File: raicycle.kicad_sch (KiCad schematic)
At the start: 8 parts, among them U1 ESP32_Feather, U2 VL53L0X, U3 BME688

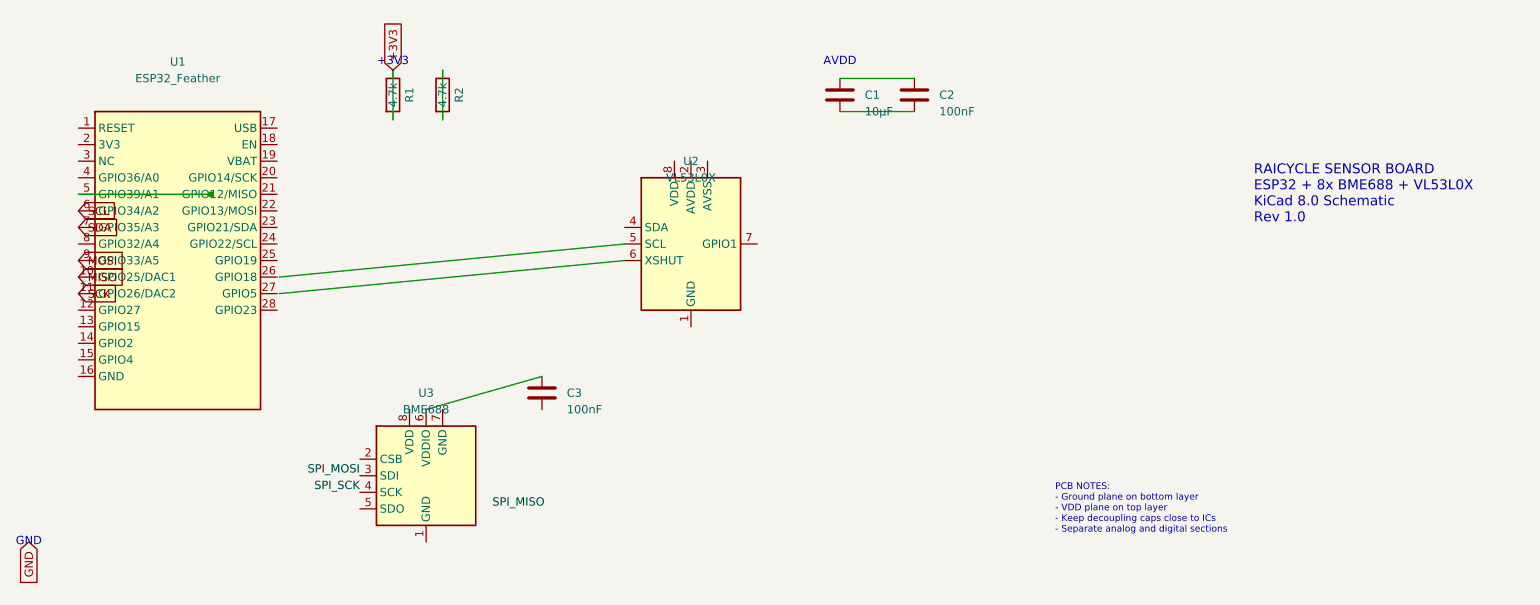
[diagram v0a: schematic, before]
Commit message: Complete KiCad 8.0 schematic implementation with all requirements
Co-authored-by: 968096 <203631091+968096@users.noreply.github.com>
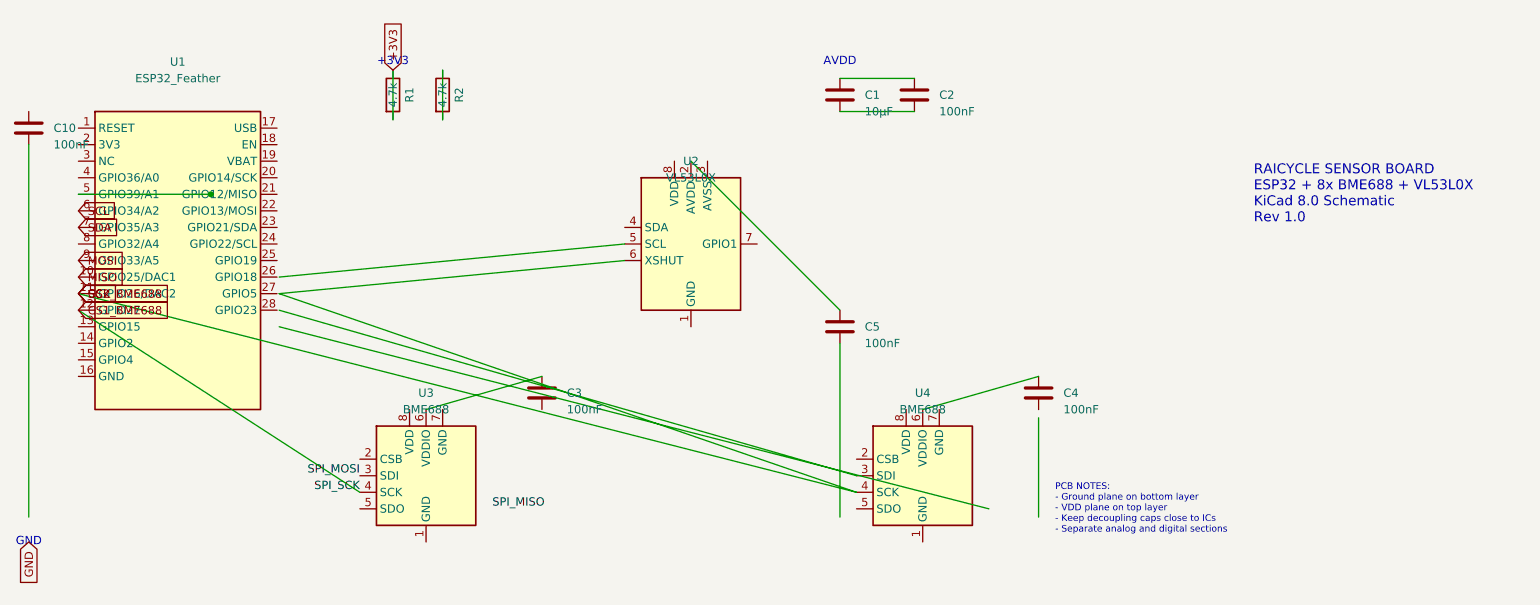
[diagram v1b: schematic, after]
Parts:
- added C10, C4, C5: 100nF, Capacitor_SMD:C_0603_1608Metric, symbol Device:C
- added U4: BME688, Package_LGA:Bosch_LGA-8_3x3mm_P0.8mm_ClockwisePinNumbering, symbol Sensor:BME688
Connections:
- net SCK is gone; now on net CS2_BME688: U1.11 (GPIO26/DAC2)
- net SPI_SCK is gone; now on net CS1_BME688: U3.4 (SCK)
- net CS1_BME688: now reaches U1.12 (GPIO27)
- net at U2.2 (AVDD): now also C5.1
- net CS2_BME688: now reaches U2.6 (XSHUT)
- net CS2_BME688: now also U4.4 (SCK)
- new net: C4.1, U4.6 (VDDIO)
